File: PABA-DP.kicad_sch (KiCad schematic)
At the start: 0 parts

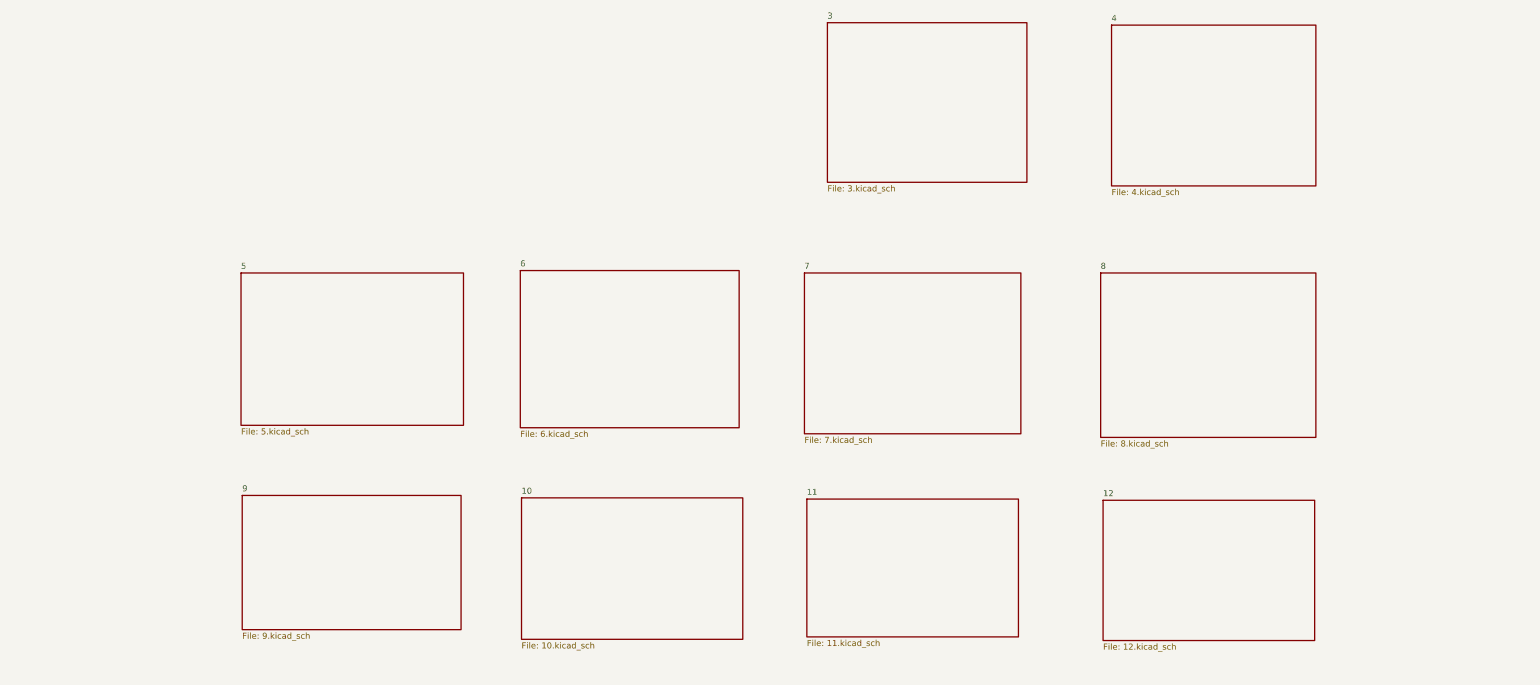
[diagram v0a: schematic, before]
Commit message: final update
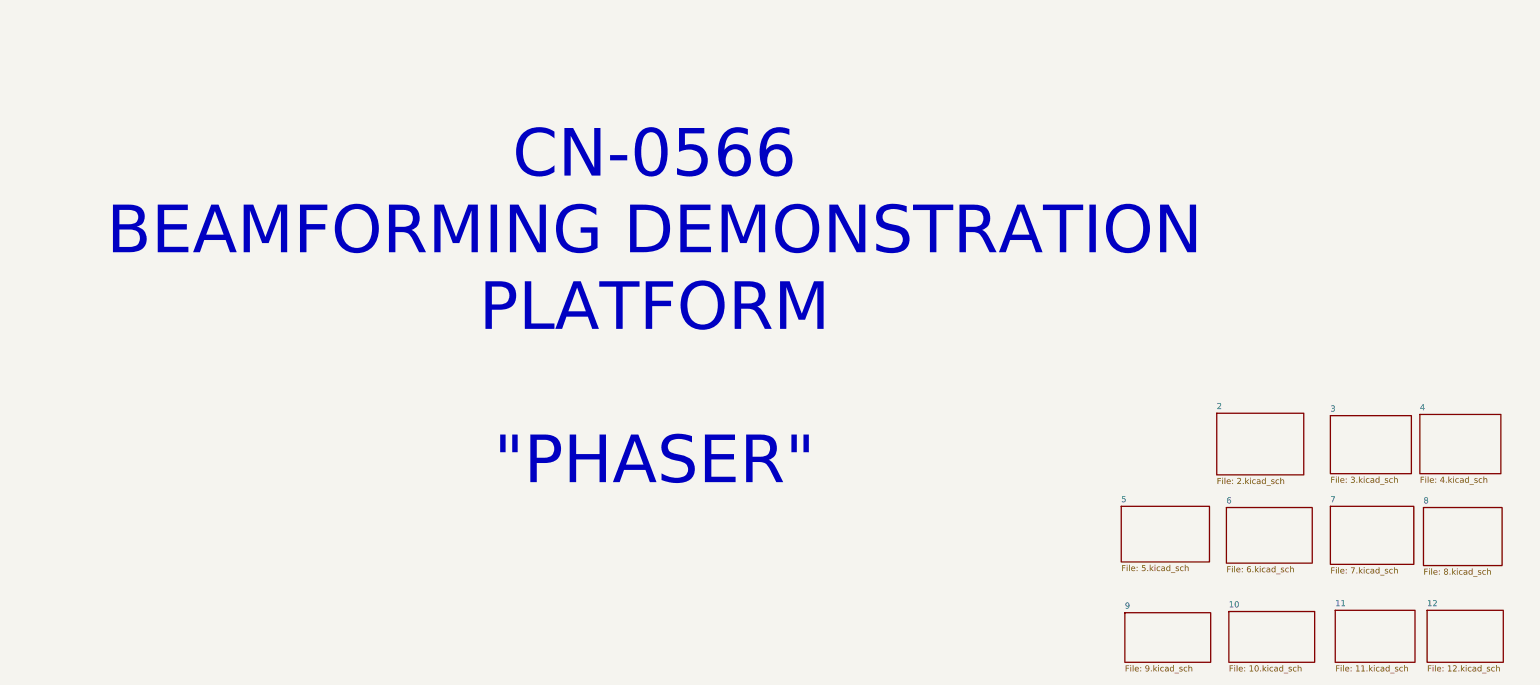
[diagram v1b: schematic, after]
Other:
- added sheet 2 (2.kicad_sch)
- note added: "CN-0566 BEAMFORMING DEMONSTRATION PLATFORM "PHASER""
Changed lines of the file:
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@@
 	(generator_version "9.0")
 	(paper "A3")
-	(sheet
-		(at 129.286 101.6)
-		(size 46.736 32.004)
+	(text "CN-0566\nBEAMFORMING DEMONSTRATION\nPLATFORM\n\n\"PHASER\""
+		(exclude_from_sim no)
+		(at 216.154 108.966 0)
+		(effects
+			(font
+				(size 10 10)
+				(thickness 1.25)
+				(color 0 0 0 1)
+			)
+		)
+	)
+	(sheet
+		(at 314.198 150.622)
+		(size 18.542 11.684)
 		(exclude_from_sim no)
 		(in_bom yes)
@@
 		)
 		(property "Sheetname" "5"
-			(at 129.286 100.8884 0)
+			(at 314.198 149.9104 0)
 			(effects
 				(font
@@
 		)
 		(property "Sheetfile" "5.kicad_sch"
-			(at 129.286 134.1886 0)
+			(at 314.198 162.8906 0)
 			(effects
 				(font
@@
 	)
 	(sheet
-		(at 312.166 49.53)
-		(size 42.926 33.782)
+		(at 376.936 131.318)
+		(size 17.018 12.446)
 		(exclude_from_sim no)
 		(in_bom yes)
@@
 		)
 		(property "Sheetname" "4"
-			(at 312.166 48.8184 0)
+			(at 376.936 130.6064 0)
 			(effects
 				(font
@@
 		)
 		(property "Sheetfile" "4.kicad_sch"
-			(at 312.166 83.8966 0)
+			(at 376.936 144.3486 0)
 			(effects
 				(font
@@
 	)
 	(sheet
-		(at 309.88 101.6)
-		(size 45.212 34.544)
+		(at 377.698 150.876)
+		(size 16.51 12.192)
 		(exclude_from_sim no)
 		(in_bom yes)
@@
 		)
 		(property "Sheetname" "8"
-			(at 309.88 100.8884 0)
+			(at 377.698 150.1644 0)
 			(effects
 				(font
@@
 		)
 		(property "Sheetfile" "8.kicad_sch"
-			(at 309.88 136.7286 0)
+			(at 377.698 163.6526 0)
 			(effects
 				(font
@@
 	)
 	(sheet
-		(at 187.96 101.092)
-		(size 45.974 33.02)
+		(at 336.296 150.876)
+		(size 18.034 11.684)
 		(exclude_from_sim no)
 		(in_bom yes)
@@
 		)
 		(property "Sheetname" "6"
-			(at 187.96 100.3804 0)
+			(at 336.296 150.1644 0)
 			(effects
 				(font
@@
 		)
 		(property "Sheetfile" "6.kicad_sch"
-			(at 187.96 134.6966 0)
+			(at 336.296 163.1446 0)
 			(effects
 				(font
@@
 	)
 	(sheet
-		(at 188.214 148.844)
-		(size 46.482 29.718)
+		(at 336.804 172.72)
+		(size 18.034 10.668)
 		(exclude_from_sim no)
 		(in_bom yes)
@@
 		)
 		(property "Sheetname" "10"
-			(at 188.214 148.1324 0)
+			(at 336.804 172.0084 0)
 			(effects
 				(font
@@
 		)
 		(property "Sheetfile" "10.kicad_sch"
-			(at 188.214 179.1466 0)
+			(at 336.804 183.9726 0)
 			(effects
 				(font
@@
 	)
 	(sheet
-		(at 248.158 149.098)
-		(size 44.45 28.956)
+		(at 359.156 172.466)
+		(size 16.764 10.922)
 		(exclude_from_sim no)
 		(in_bom yes)
@@
 		)
 		(property "Sheetname" "11"
-			(at 248.158 148.3864 0)
+			(at 359.156 171.7544 0)
 			(effects
 				(font
@@
 		)
 		(property "Sheetfile" "11.kicad_sch"
-			(at 248.158 178.6386 0)
+			(at 359.156 183.9726 0)
 			(effects
 				(font
@@
 	)
 	(sheet
-		(at 129.54 148.336)
-		(size 45.974 28.194)
+		(at 314.96 172.974)
+		(size 18.034 10.414)
 		(exclude_from_sim no)
 		(in_bom yes)
@@
 		)
 		(property "Sheetname" "9"
-			(at 129.54 147.6244 0)
+			(at 314.96 172.2624 0)
 			(effects
 				(font
@@
 		)
 		(property "Sheetfile" "9.kicad_sch"
-			(at 129.54 177.1146 0)
+			(at 314.96 183.9726 0)
 			(effects
 				(font
@@
 	)
 	(sheet
-		(at 310.388 149.352)
-		(size 44.45 29.464)
+		(at 378.46 172.466)
+		(size 16.002 10.922)
 		(exclude_from_sim no)
 		(in_bom yes)
@@
 		)
 		(property "Sheetname" "12"
-			(at 310.388 148.6404 0)
+			(at 378.46 171.7544 0)
 			(effects
 				(font
@@
 		)
 		(property "Sheetfile" "12.kicad_sch"
-			(at 310.388 179.4006 0)
+			(at 378.46 183.9726 0)
 			(effects
 				(font
@@
 	)
 	(sheet
-		(at 252.476 49.022)
-		(size 41.91 33.528)
+		(at 358.14 131.572)
+		(size 17.018 12.192)
 		(exclude_from_sim no)
 		(in_bom yes)
@@
 		)
 		(property "Sheetname" "3"
-			(at 252.476 48.3104 0)
+			(at 358.14 130.8604 0)
 			(effects
 				(font
@@
 		)
 		(property "Sheetfile" "3.kicad_sch"
-			(at 252.476 83.1346 0)
+			(at 358.14 144.3486 0)
 			(effects
 				(font
@@
 	)
 	(sheet
-		(at 247.65 101.6)
-		(size 45.466 33.782)
+		(at 334.264 131.064)
+		(size 18.288 12.954)
+		(exclude_from_sim no)
+		(in_bom yes)
+		(on_board yes)
+		(dnp no)
+		(fields_autoplaced yes)
+		(stroke
+			(width 0.1524)
+			(type solid)
+		)
+		(fill
+			(color 0 0 0 0.0000)
+		)
+		(property "Sheetname" "2"
+			(at 334.264 130.3524 0)
+			(effects
+				(font
+					(size 1.27 1.27)
+				)
+				(justify left bottom)
+			)
+		)
+		(property "Sheetfile" "2.kicad_sch"
+			(at 334.264 144.6026 0)
+			(effects
+				(font
+					(size 1.27 1.27)
+				)
+				(justify left top)
+			)
+		)
+		(instances
+			(project "PABA-DP"
+				(path "/1b74eff2-580c-4b71-b276-daaf48eb9de6"
+					(page "2")
+				)
+			)
+		)
+	)
+	(sheet
+		(at 358.14 150.622)
+		(size 17.526 12.192)
 		(exclude_from_sim no)
 		(in_bom yes)
@@
 		)
 		(property "Sheetname" "7"
-			(at 247.65 100.8884 0)
+			(at 358.14 149.9104 0)
 			(effects
 				(font
@@
 		)
 		(property "Sheetfile" "7.kicad_sch"
-			(at 247.65 135.9666 0)
-			(effects
-				(font
+			(at 358.14 163.3986 0)
+			(effects
+				(font
